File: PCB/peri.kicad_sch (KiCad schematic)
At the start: 6 parts, among them J1 Micro_SD_Card, J5 BT USB Debug, J6 SPI Debug, J7 UART Debug, U4 RN42, U8 362 TFT LCD

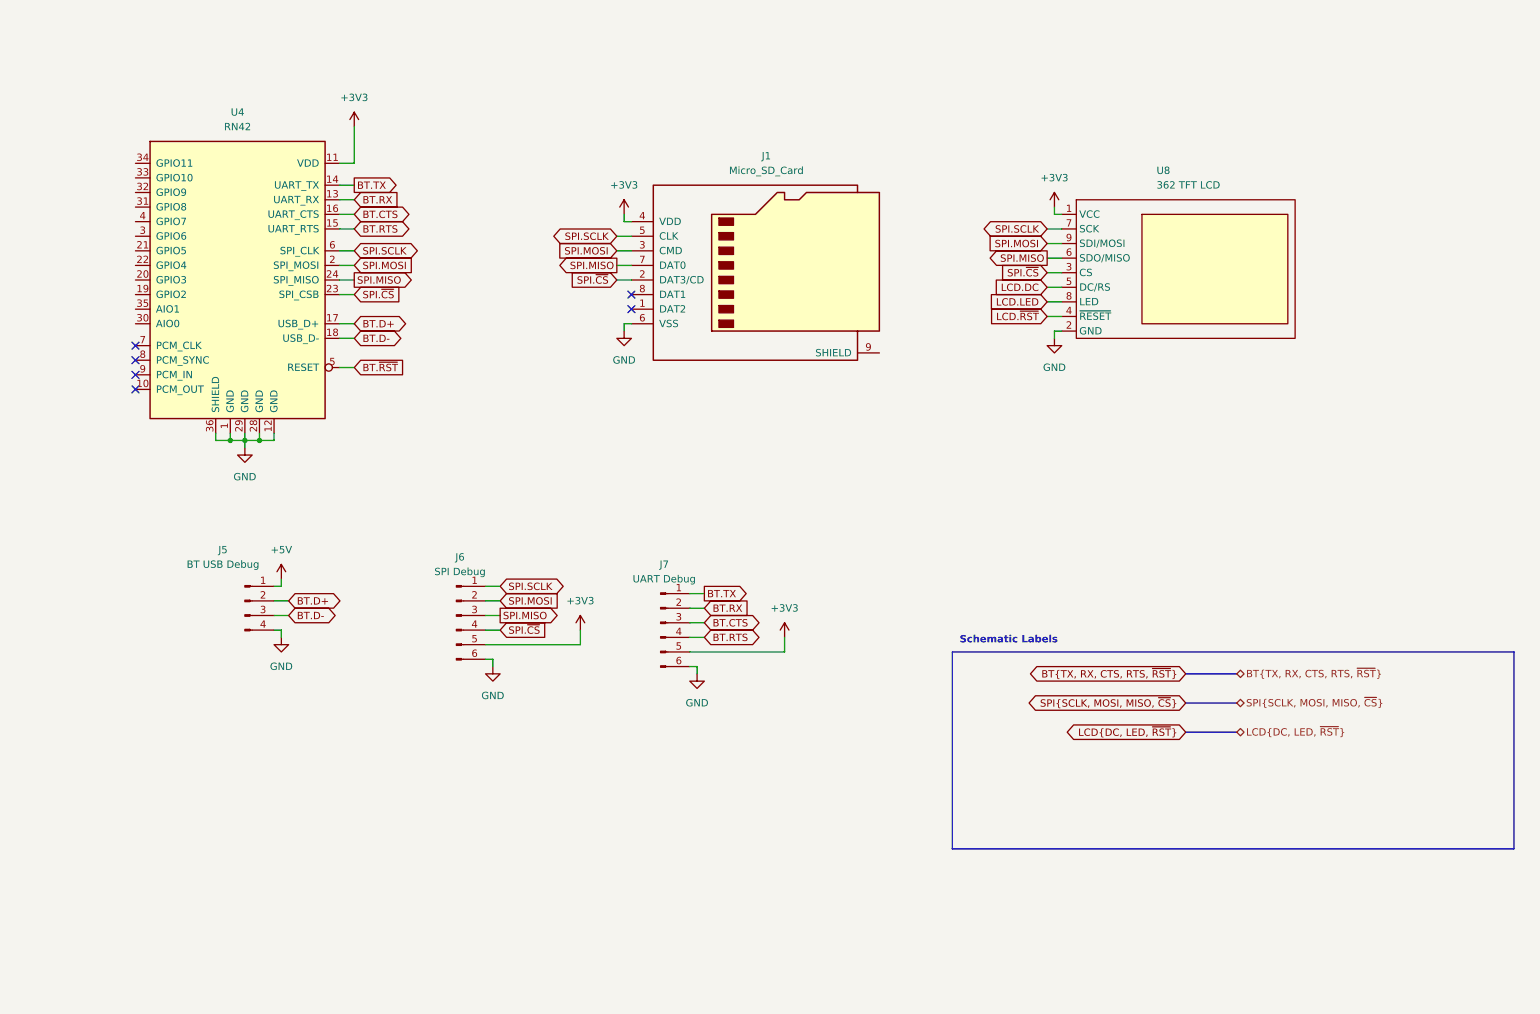
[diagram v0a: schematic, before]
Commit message: PCB Update - Minh
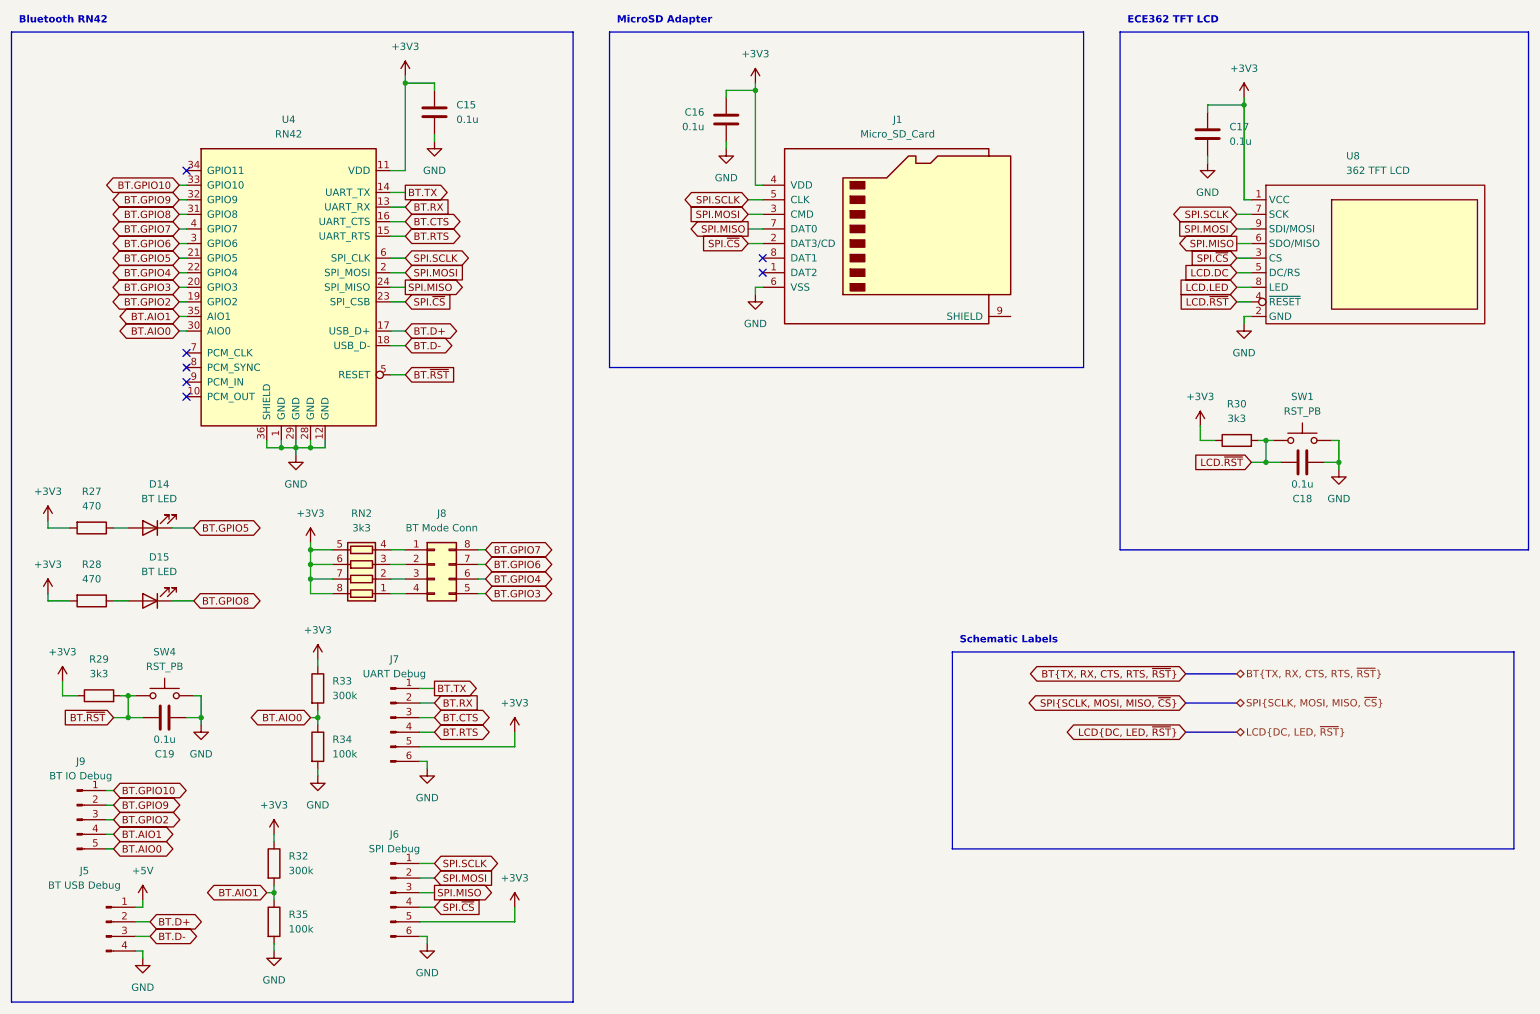
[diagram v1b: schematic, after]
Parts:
- added C15, C16, C17, C18, C19: 0.1u, symbol Device:C
- added D14, D15: BT LED, symbol Device:LED
- added J8: BT Mode Conn, symbol Connector_Generic:Conn_02x04_Counter_Clockwise
- added J9: BT IO Debug, symbol Connector:Conn_01x05_Pin
- added R27, R28: 470, symbol Device:R
- added R29, R30: 3k3, symbol Device:R
- added R32, R33: 300k, symbol Device:R
- added R34, R35: 100k, symbol Device:R
- added RN2: 3k3, symbol Device:R_Pack04
- added SW1, SW4: RST_PB, symbol Switch:SW_Push
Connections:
- net +3V3: now also C15.1, C16.1, C17.1, R27.2, R28.2, R29.1, R30.1, R32.1, R33.1, RN2.5 (R4.2), RN2.6 (R3.2), RN2.7 (R2.2), RN2.8 (R1.2)
- net BT.~{RST}: now also C19.2, R29.2, SW4.1
- net GND: now also C15.2, C16.2, C17.2, C18.1, C19.1, R34.2, R35.2, SW1.2, SW4.2
- net LCD.~{RST}: now also C18.2, R30.2, SW1.1
- net BT.GPIO2: now reaches U4.19 (GPIO2)
- net BT.GPIO2: now also J9.3 (Pin_3)
- net BT.GPIO3: now reaches U4.20 (GPIO3)
- net BT.GPIO3: now also J8.5 (Pin_5)
- net BT.GPIO5: now reaches U4.21 (GPIO5)
- net BT.GPIO5: now also D14.1 (K)
- net BT.GPIO4: now reaches U4.22 (GPIO4)
- net BT.GPIO4: now also J8.6 (Pin_6)
- net BT.GPIO6: now reaches U4.3 (GPIO6)
- net BT.GPIO6: now also J8.7 (Pin_7)
- net BT.AIO0: now reaches U4.30 (AIO0)
- net BT.AIO0: now also J9.5 (Pin_5), R33.2, R34.1
- net BT.GPIO8: now reaches U4.31 (GPIO8)
- net BT.GPIO8: now also D15.1 (K)
- net BT.GPIO9: now reaches U4.32 (GPIO9)
- net BT.GPIO9: now also J9.2 (Pin_2)
- net BT.GPIO10: now reaches U4.33 (GPIO10)
- net BT.GPIO10: now also J9.1 (Pin_1)
- net BT.AIO1: now reaches U4.35 (AIO1)
- net BT.AIO1: now also J9.4 (Pin_4), R32.2, R35.1
- net BT.GPIO7: now reaches U4.4 (GPIO7)
- net BT.GPIO7: now also J8.8 (Pin_8)
- new net: J8.1 (Pin_1), RN2.4 (R4.1)
- new net: J8.2 (Pin_2), RN2.3 (R3.1)
- new net: J8.3 (Pin_3), RN2.2 (R2.1)
- new net: J8.4 (Pin_4), RN2.1 (R1.1)
- new net: D14.2 (A), R27.1
- new net: D15.2 (A), R28.1
- no-connect marks 6 -> 7
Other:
- note added: "Bluetooth RN42"
- note added: "ECE362 TFT LCD"
- note added: "MicroSD Adapter"
- moved on the sheet: J1, J5, J6, J7, U4
